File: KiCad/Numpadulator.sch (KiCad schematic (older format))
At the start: 42 parts, among them U1 PRO_MICRO_C

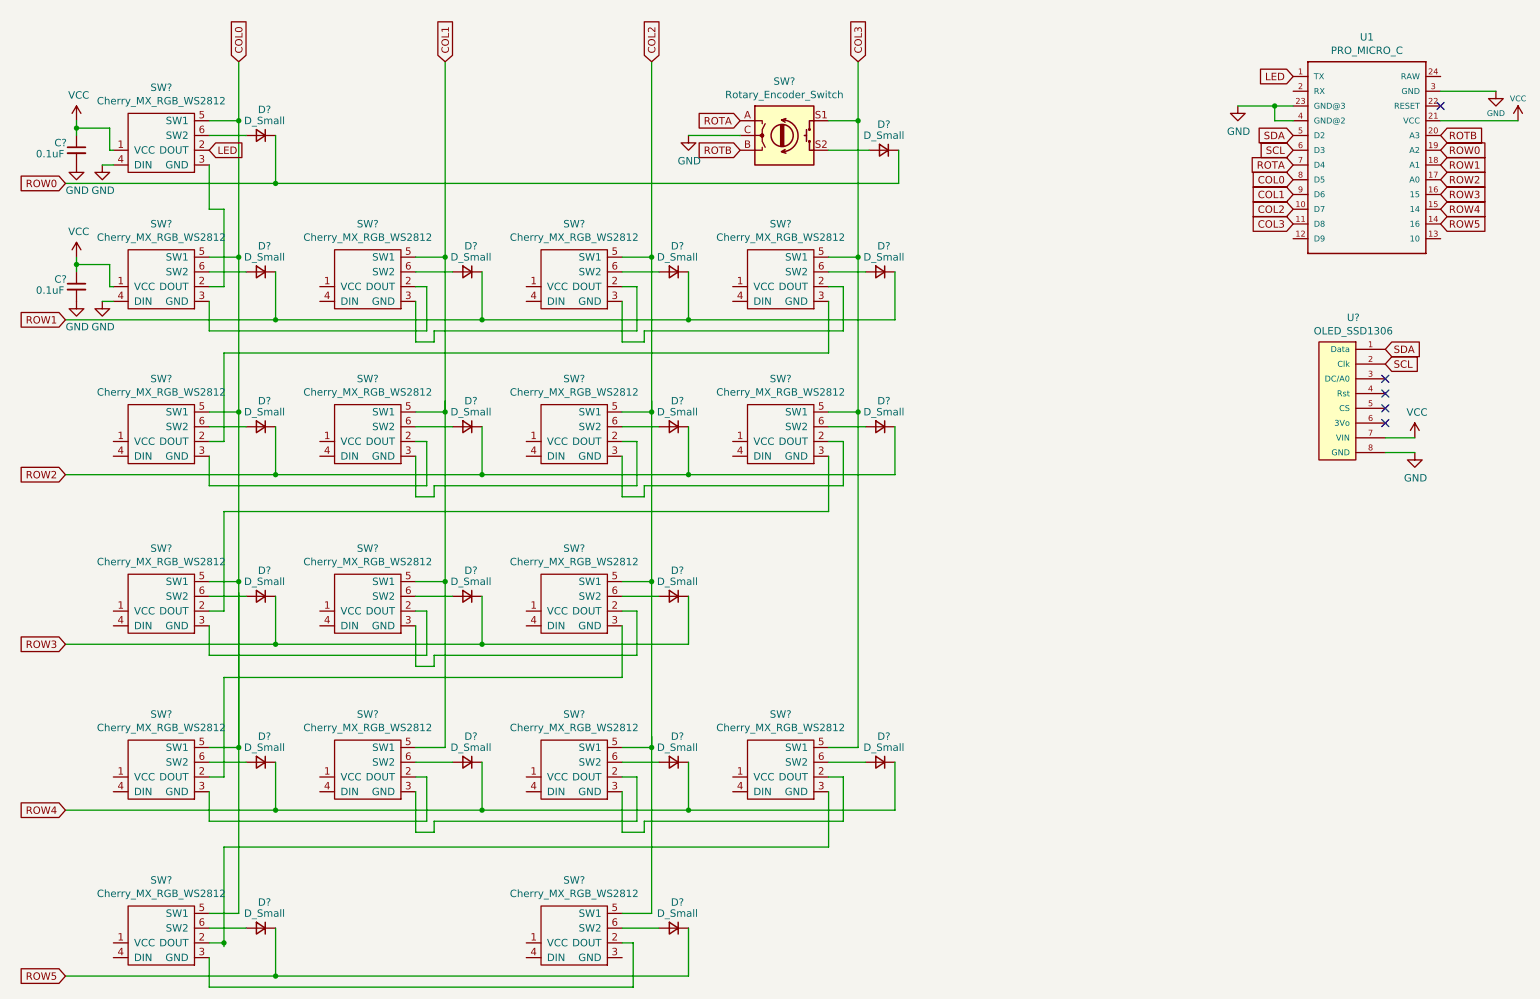
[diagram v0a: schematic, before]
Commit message: Started to make look better
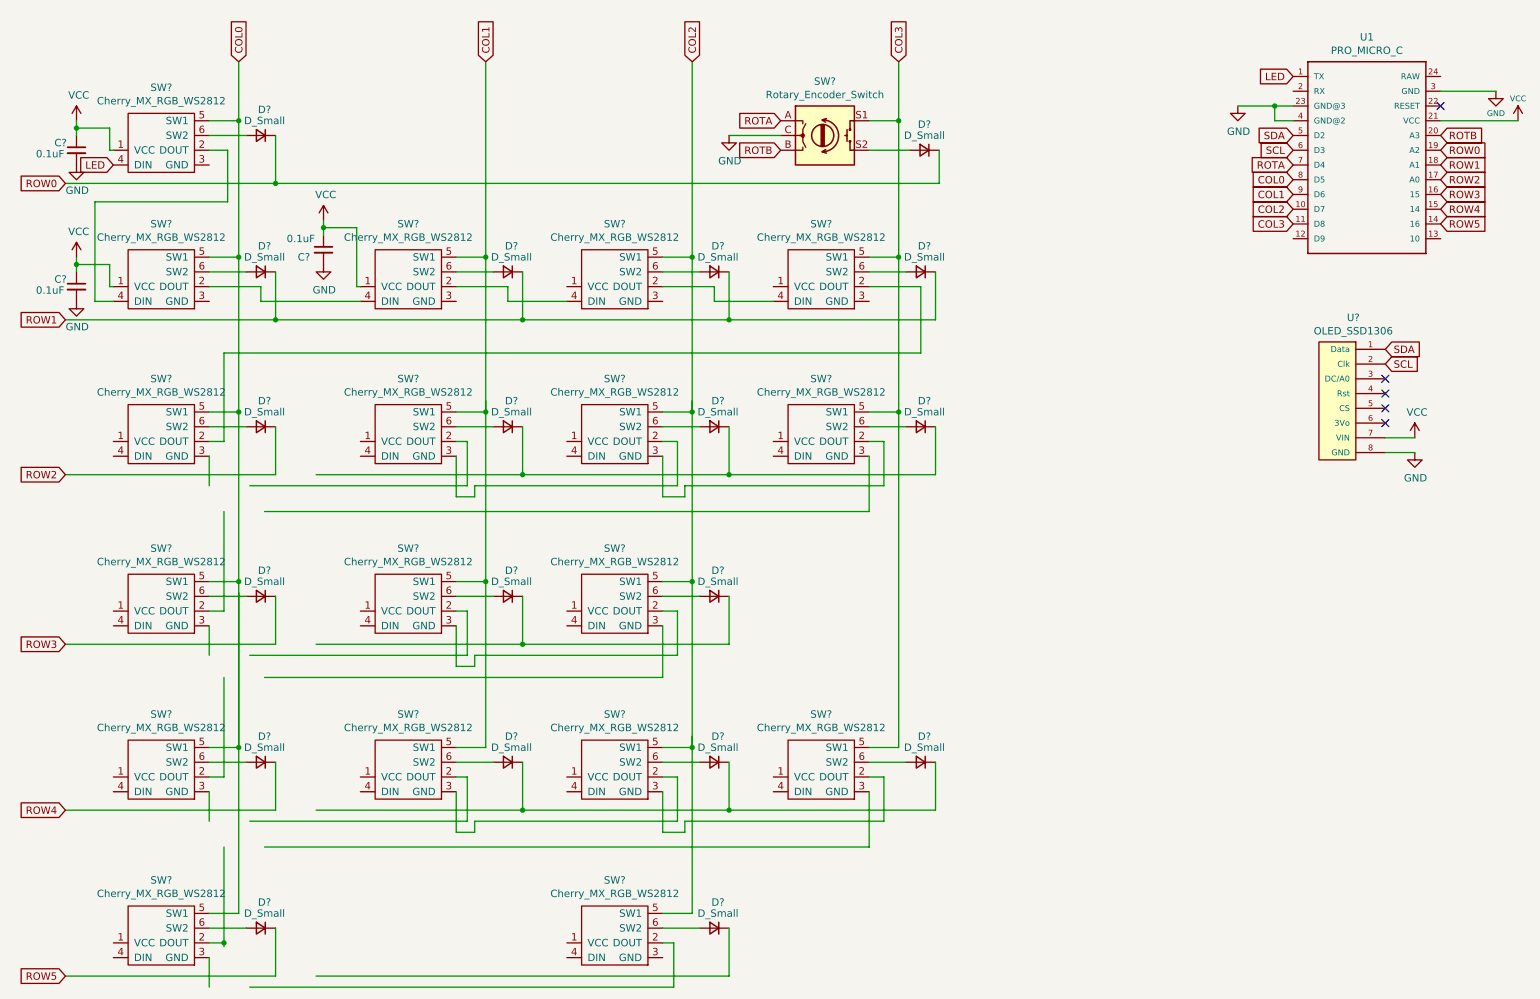
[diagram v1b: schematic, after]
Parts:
- added C?: 0.1uF, symbol Device:C_Small
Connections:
- wire segments 203 -> 201
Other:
- moved on the sheet: D?, SW?
